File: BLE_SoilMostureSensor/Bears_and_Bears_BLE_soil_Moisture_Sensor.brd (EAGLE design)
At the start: 33.6 x 76.2 mm, 50 parts, among them Q1 2N3904, U2 EFR32BG13, X1 20317

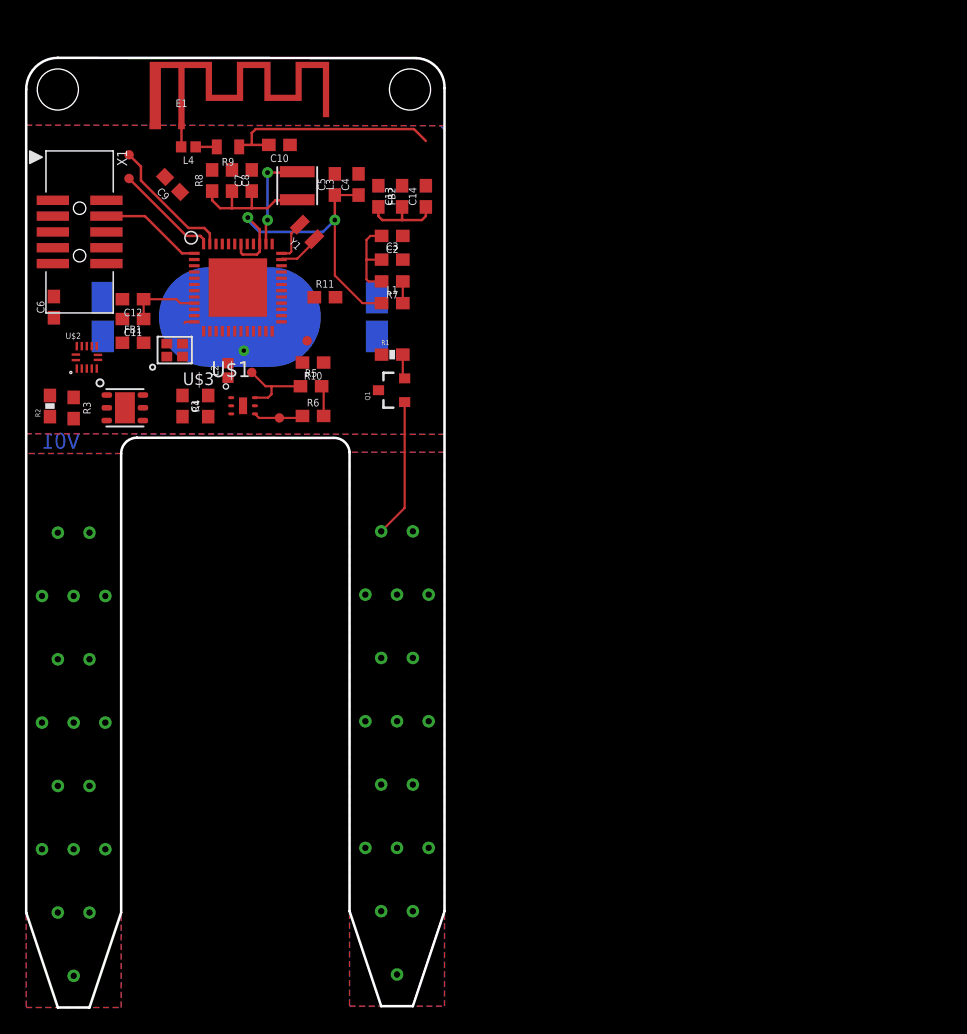
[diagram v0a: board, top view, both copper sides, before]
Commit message: first prototype
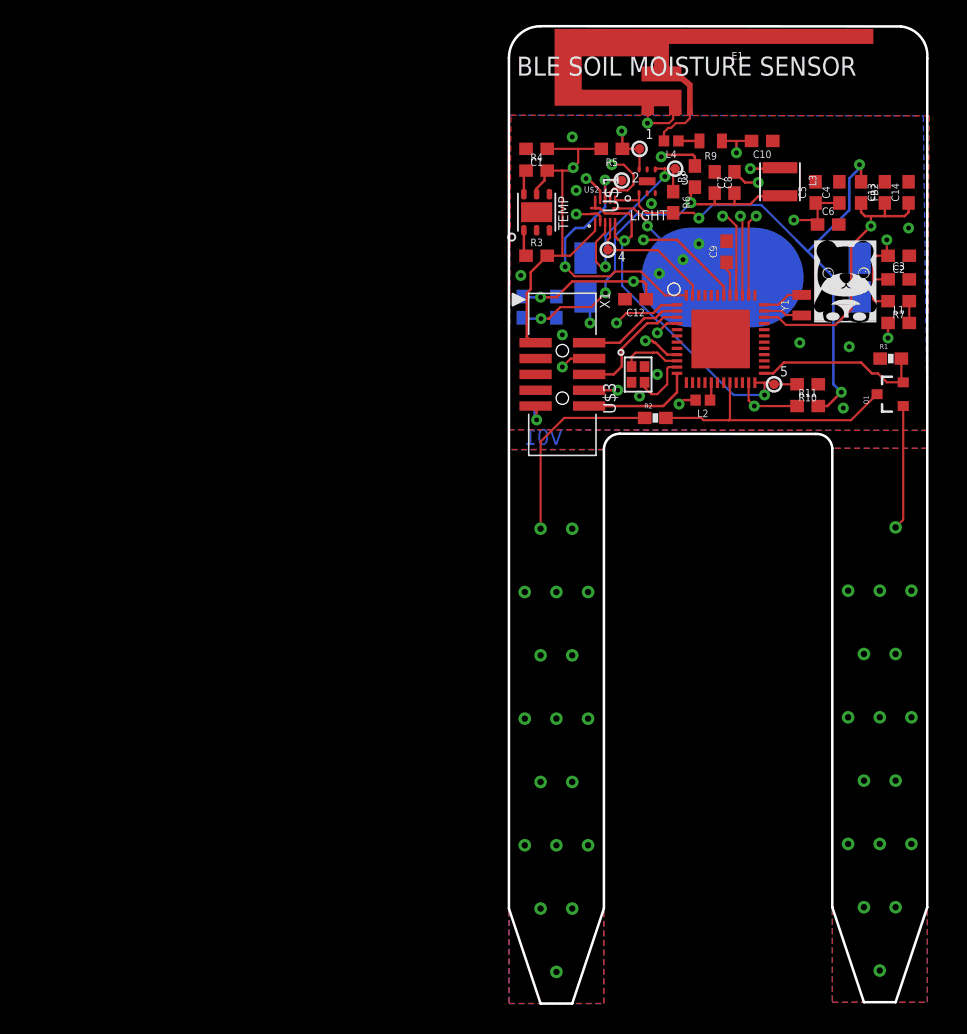
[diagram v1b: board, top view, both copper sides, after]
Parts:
- removed STANDOFF1, STANDOFF2: STAND-OFF, SparkFun-Electromechanical:STAND-OFF
- added U$4: IMAGES#JPG, images#jpg(2):IMAGES#JPG
- E1: value ANTENNA-GROUNDEDTRACE-15.2MM -> ANTENNA-GROUNDEDTRACE-25.7MM; device SparkFun-RF:TRACE_ANTENNA_2.4GHZ_15.2MM -> SparkFun-RF:TRACE_ANTENNA_2.4GHZ_25.7MM
- moved FRAME2 107.9 mm to (59.1, -8.57)
- moved C6 62.5 mm to (64.4, 62.8), turned to 0 degrees
- moved R2 48.6 mm to (50.5, 47.3), turned to 0 degrees
- moved C9 44.8 mm to (56.2, 60.6), turned to 90 degrees
- moved U$2 43.2 mm to (45.4, 62.9)
- moved E1 40.8 mm to (53.3, 71.6)
- moved C2 40.7 mm to (70.0, 60.3)
- moved C3 40.7 mm to (70.0, 58.4)
- moved L1 40.7 mm to (70.0, 54.9)
- moved R7 40.7 mm to (70.0, 56.7)
- moved X1 40.4 mm to (43.0, 50.8)
- moved C12 40.3 mm to (48.9, 56.8)
- moved Y1 40.1 mm to (62.2, 56.4), turned to 90 degrees
- moved Q1 40.0 mm to (69.4, 49.2)
- moved R1 40.0 mm to (69.4, 52.1)
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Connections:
- removed net N$2: U2.14, U2.15, U2.37, U2.GND
- net GND: now also E1.GND2, U2.14, U2.15, U2.37, U2.GND
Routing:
- net VDD: track 2.45 -> 87.9 mm, vias 0 -> 4
- net PAVDD: track 6.60 -> 50.9 mm, vias 0 -> 2
- net SENSOR_ENABLE: track 0.00 -> 31.7 mm, vias 0 -> 2
- net V_BATT: track 26.6 -> 57.3 mm, vias 2 -> 7
- net GND_DETECT: track 0.00 -> 25.6 mm, vias 0 -> 2
- net AVDD: track 7.01 -> 29.4 mm, vias 0 -> 2
- net SOIL_MOIST_PWR: track 0.00 -> 20.9 mm
- net VDCDC: track 10.9 -> 30.3 mm, vias 0 -> 3
- net GND: track 0.00 -> 17.0 mm, vias 0 -> 17
- net PROBE2: track 0.00 -> 16.1 mm
- net RFVDD: track 5.78 -> 21.4 mm, vias 0 -> 3
- net SDA: track 8.38 -> 22.6 mm, vias 0 -> 2
- net SCL_IN: track 4.02 -> 18.1 mm, vias 0 -> 2
- net SIG: track 1.97 -> 14.2 mm
- net TDI: track 0.00 -> 10.3 mm, vias 0 -> 2
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- added copper zone on layer 2, net GND
- added copper zone on layer 15, net V_BATT
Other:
- board size 33.6 x 76.2 mm -> 33.6 x 78.4 mm
- board text added: "1"
- board text added: "2"
- board text added: "3"
- board text added: "4"
- board text added: "5"
- board text added: "BLE SOIL MOISTURE SENSOR"
- board text added: "LIGHT"
- board text added: "TEMP"
